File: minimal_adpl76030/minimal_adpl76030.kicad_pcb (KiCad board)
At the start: 4 copper layers, 30.5 x 21.6 mm, 26 parts, among them Q1 60 V, Q2 60 V, Q3 25 V, Q4 25 V, U1 ADPL76030EUFD-PBF

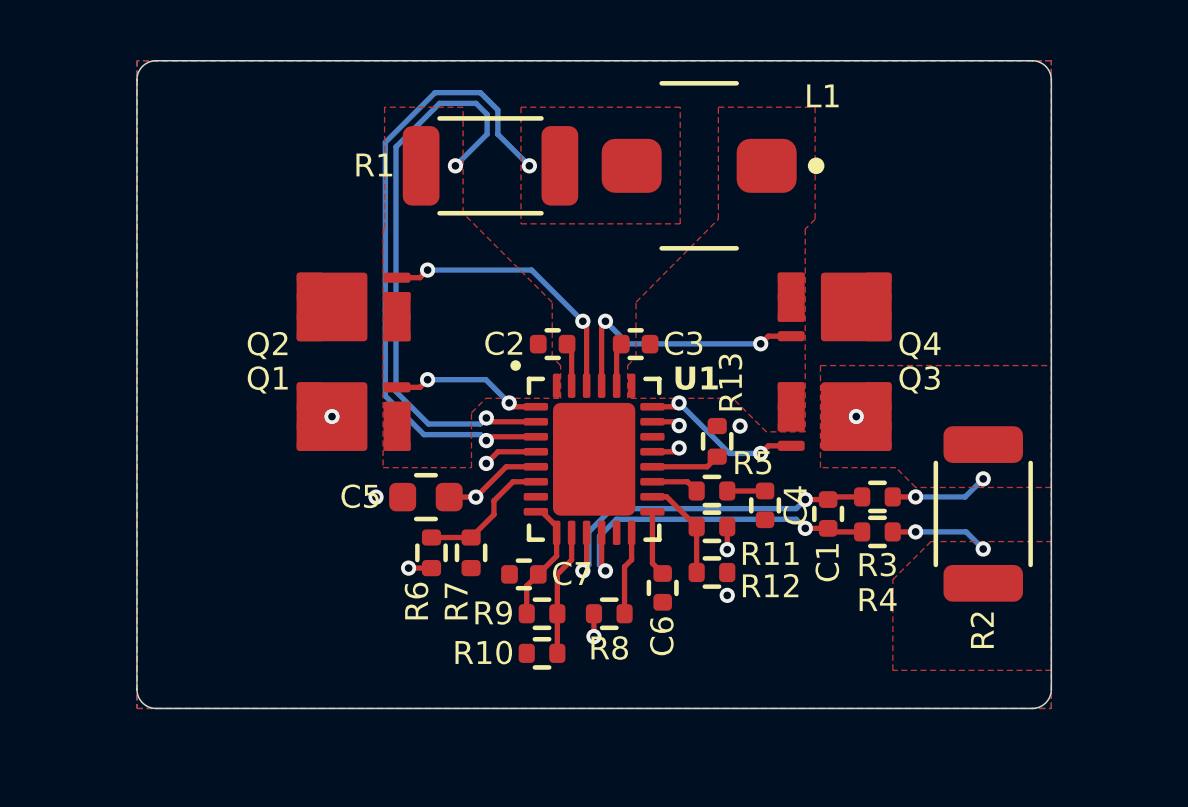
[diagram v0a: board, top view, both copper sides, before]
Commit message: backup
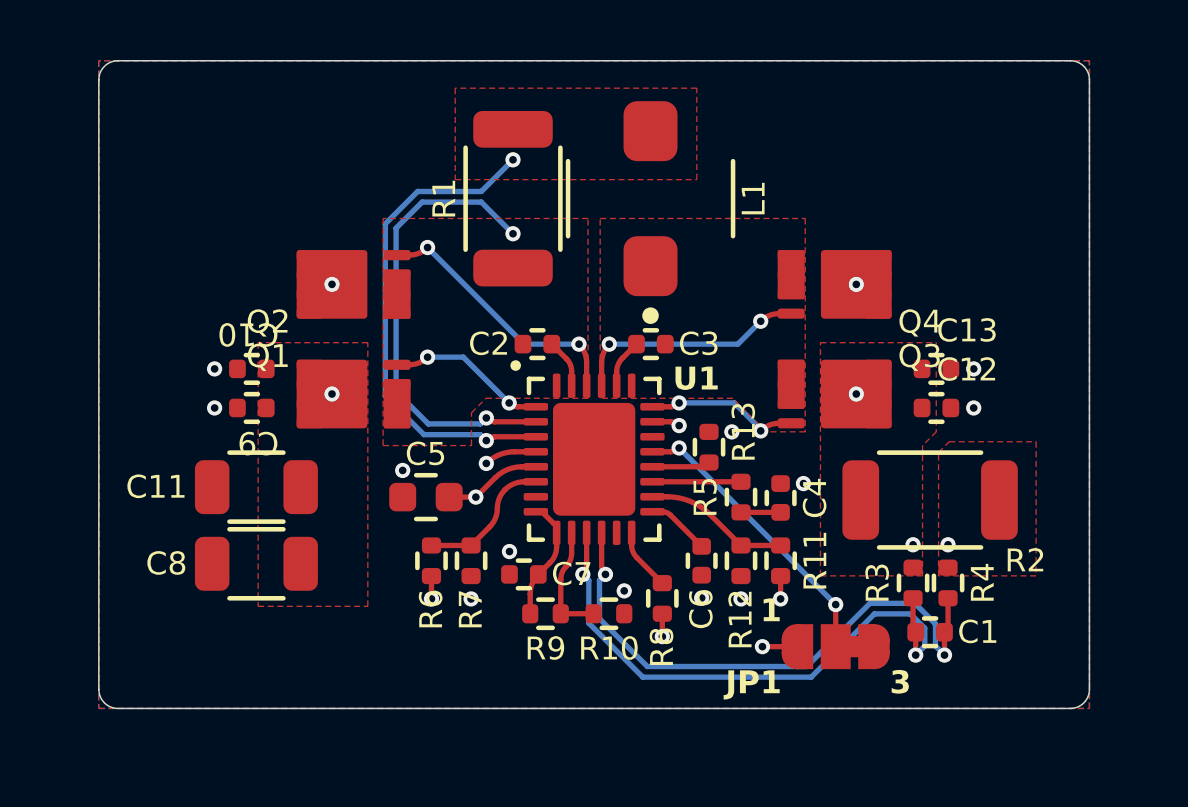
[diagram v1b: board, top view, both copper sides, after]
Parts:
- added C10: 100 nF, capacitor_footprints:C_0402_1005Metric, F.Cu at (128.5, 88.0)
- added C11: 4.7 µF, capacitor_footprints:C_1206_3216Metric, F.Cu at (128.7, 92.0)
- added C12: 100 nF, capacitor_footprints:C_0402_1005Metric, F.Cu at (151.4, 89.3)
- added C13: 100 nF, capacitor_footprints:C_0402_1005Metric, F.Cu at (151.4, 88.0)
- added C8: 4.7 µF, capacitor_footprints:C_1206_3216Metric, F.Cu at (128.7, 94.5)
- added C9: 100 nF, capacitor_footprints:C_0402_1005Metric, F.Cu at (128.5, 89.3)
- added JP1: SolderJumper_3_Open, solder_jumper_footprints:SolderJumper-3_P1.3mm_Bridged_2_3_RoundedPad1.0x1.5mm_NumberLabels_1, F.Cu at (148.0, 97.3)
- moved C1 5.21 mm to (151.2, 96.8), turned to 0 degrees
- moved R3 3.10 mm to (150.6, 95.2), turned to -90 degrees
- moved R4 2.90 mm to (151.8, 95.2), turned to -90 degrees
- moved R10 2.59 mm to (140.4, 96.2), turned to 0 degrees
- moved R11 2.55 mm to (146.2, 94.4), turned to 90 degrees
- moved L1 1.96 mm to (141.8, 82.4), turned to 90 degrees
- moved R8 1.84 mm to (142.2, 95.7), turned to -90 degrees
- moved R2 1.83 mm to (151.2, 92.4), turned to 0 degrees
- moved C6 1.58 mm to (143.5, 94.4)
- moved R1 1.33 mm to (137.2, 82.4), turned to 90 degrees
- moved R12 1.04 mm to (144.8, 94.4), turned to 90 degrees
- moved R5 0.99 mm to (144.8, 92.3), turned to -90 degrees
- moved Q1 0.75 mm to (131.9, 88.9)
- moved Q2 0.75 mm to (131.9, 85.2)
- moved Q3 0.75 mm to (148.0, 88.9)
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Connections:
- net Net-(U1-RT) renamed /RT
- net Net-(U1-VC) renamed /VC
- U1 pad 19: unconnected-(U1-SYNC/SPRD-Pad19) -> /SYNC/SPRD
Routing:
- net /SYNC/SPRD: track 0.00 -> 9.71 mm, vias 0 -> 2
- net /ISN: track 11.7 -> 19.1 mm
- net /ISP: track 12.3 -> 19.1 mm
- net /LSN: track 21.1 -> 16.5 mm
- net /LSP: track 19.3 -> 15.4 mm
- net /VOUT: track 4.21 -> 0.92 mm, vias 4 -> 3
- net /V_OUT: track 4.01 -> 0.76 mm, vias 3 -> 2
- net /FB: track 3.41 -> 4.85 mm
- net /VC: track 1.60 -> 2.95 mm
- net /INTVCC: track 4.07 -> 5.15 mm, vias 2 -> 3
- net unconnected-(U1-SYNC/SPRD-Pad19): track 0.94 -> 0.00 mm, vias 1 -> 0
- net /BG2: track 8.81 -> 7.89 mm
- net /~{PGOOD}: track 2.80 -> 2.07 mm
- net GND: vias 3 -> 14
- added copper zone on F.Cu, net /VIN
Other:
- board size 30.5 x 21.6 mm -> 33 x 21.6 mm

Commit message: backup
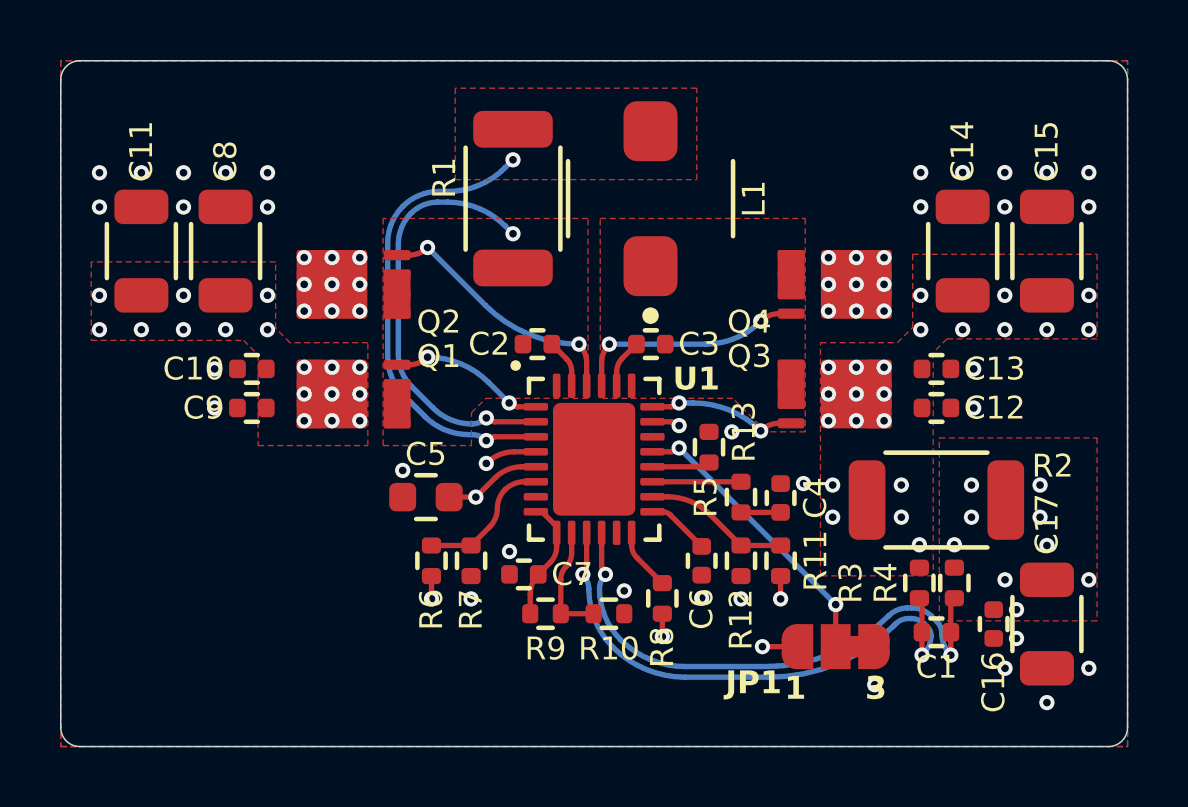
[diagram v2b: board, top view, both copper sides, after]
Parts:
- added C14: 22 µF, capacitor_footprints:C_1206_3216Metric, F.Cu at (152.2, 84.1)
- added C15: 22 µF, capacitor_footprints:C_1206_3216Metric, F.Cu at (155.0, 84.1)
- added C16: 100 nF, capacitor_footprints:C_0402_1005Metric, F.Cu at (153.3, 96.6)
- added C17: 22 µF, capacitor_footprints:C_1206_3216Metric, F.Cu at (155.0, 96.6)
- moved C8 10.5 mm to (127.7, 84.1), turned to 90 degrees
- moved C11 8.75 mm to (124.9, 84.1), turned to 90 degrees
- moved R4 0.21 mm to (152.0, 95.2)
- moved C1 0.21 mm to (151.4, 96.8)
- moved R2 0.21 mm to (151.4, 92.4)
- moved R3 0.21 mm to (150.8, 95.2)
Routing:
- net /LSN: track 16.5 -> 15.6 mm
- net /LSP: track 15.4 -> 14.4 mm
- net /ISN: track 19.1 -> 18.4 mm
- net /ISP: track 19.1 -> 18.4 mm
- net GND: vias 14 -> 51
- net /V_OUT: vias 2 -> 10
- net /VOUT: vias 3 -> 23
- net /VIN: vias 3 -> 19
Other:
- board size 33 x 21.6 mm -> 35.6 x 22.9 mm
